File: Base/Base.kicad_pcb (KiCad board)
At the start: 2 copper layers, 0 parts

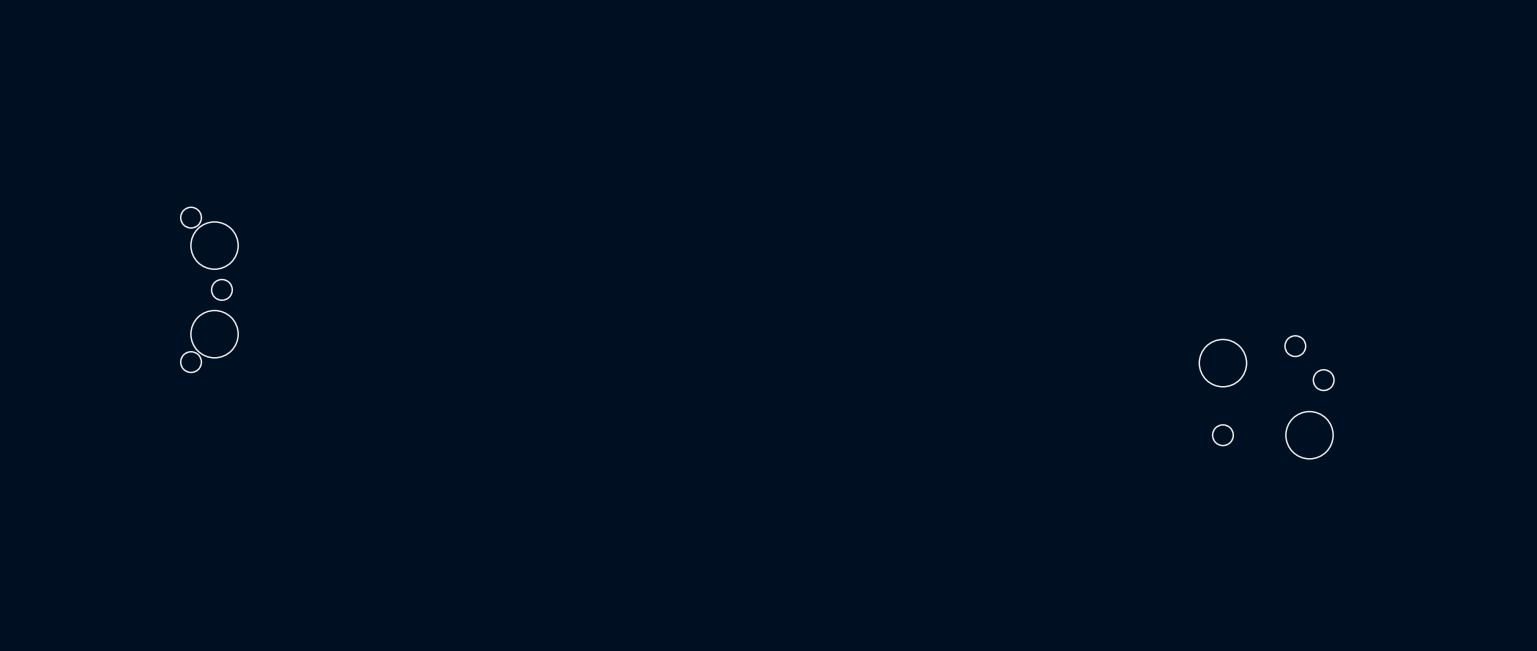
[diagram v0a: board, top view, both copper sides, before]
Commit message: add components
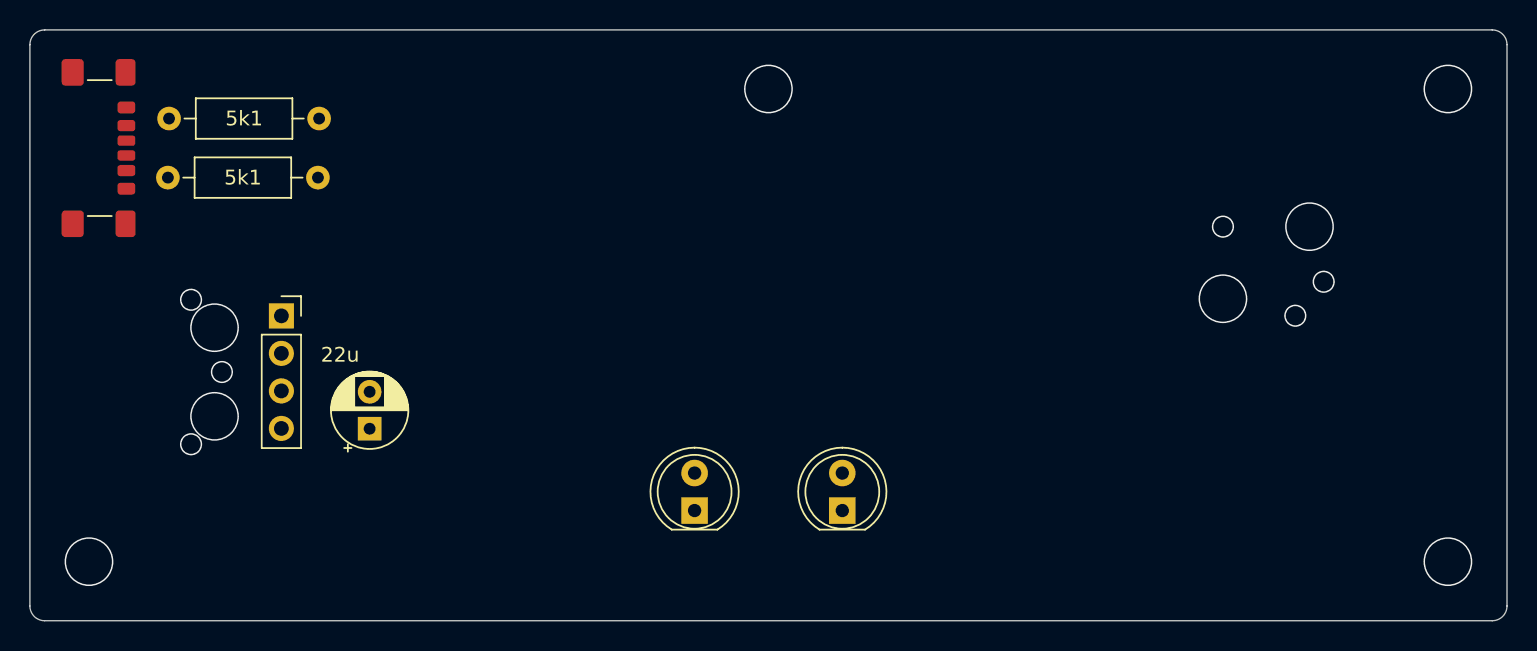
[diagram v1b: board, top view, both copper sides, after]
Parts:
- added C1: 22u, Capacitor_THT:CP_Radial_D5.0mm_P2.50mm, F.Cu at (103.0, 97.0)
- added D1: LED, LED_THT:LED_D5.0mm_Clear, F.Cu at (135.0, 102.5)
- added D2: LED, LED_THT:LED_D5.0mm_Clear, F.Cu at (125.0, 102.5)
- added J1: USB_C_Receptacle_PowerOnly_6P, Connector_USB:USB_C_Receptacle_GCT_USB4135-GF-A_6P_TopMnt_Horizontal, F.Cu at (83.5, 78.0)
- added J2: Conn_01x04_Socket, Connector_PinSocket_2.54mm:PinSocket_1x04_P2.54mm_Vertical, F.Cu at (97.0, 89.4)
- added R1: 5k1, Resistor_THT:R_Axial_DIN0207_L6.3mm_D2.5mm_P10.16mm_Horizontal, F.Cu at (89.3, 80.0)
- added R2: 5k1, Resistor_THT:R_Axial_DIN0207_L6.3mm_D2.5mm_P10.16mm_Horizontal, F.Cu at (89.4, 76.0)
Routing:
- net (no net): vias 10 -> 14
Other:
- board outline added: 100 x 40 mm
